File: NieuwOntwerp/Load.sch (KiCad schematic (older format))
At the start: 74 parts, among them J1 Conn_01x02, J2 Conn_01x02, J3 Conn_01x05, J4 Conn_01x03, J5 Conn_01x02, Q1 IRF840, Q2 IRF840, T1 EE13, U1 ESP12E, U10 MCP4725A0, U2 LNK364D, U3 LM358, U4 PC817, U5 TL431, U6 LM1117-3.3, U7 LM358

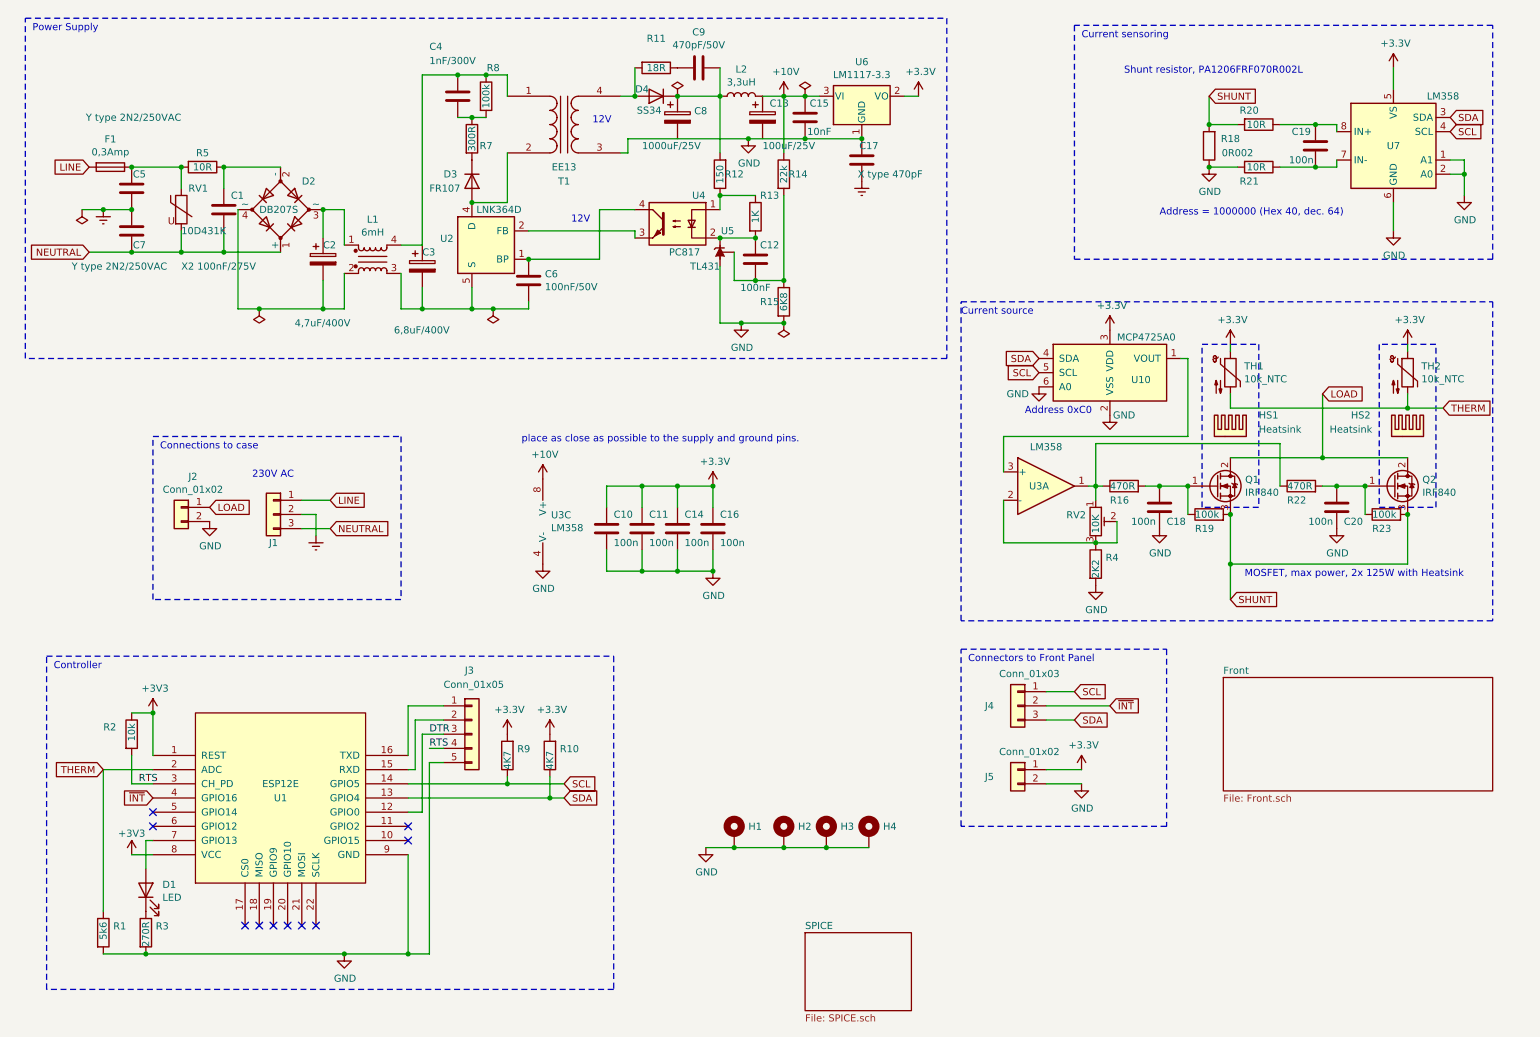
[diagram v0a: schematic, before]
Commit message: Sync_21-04-27
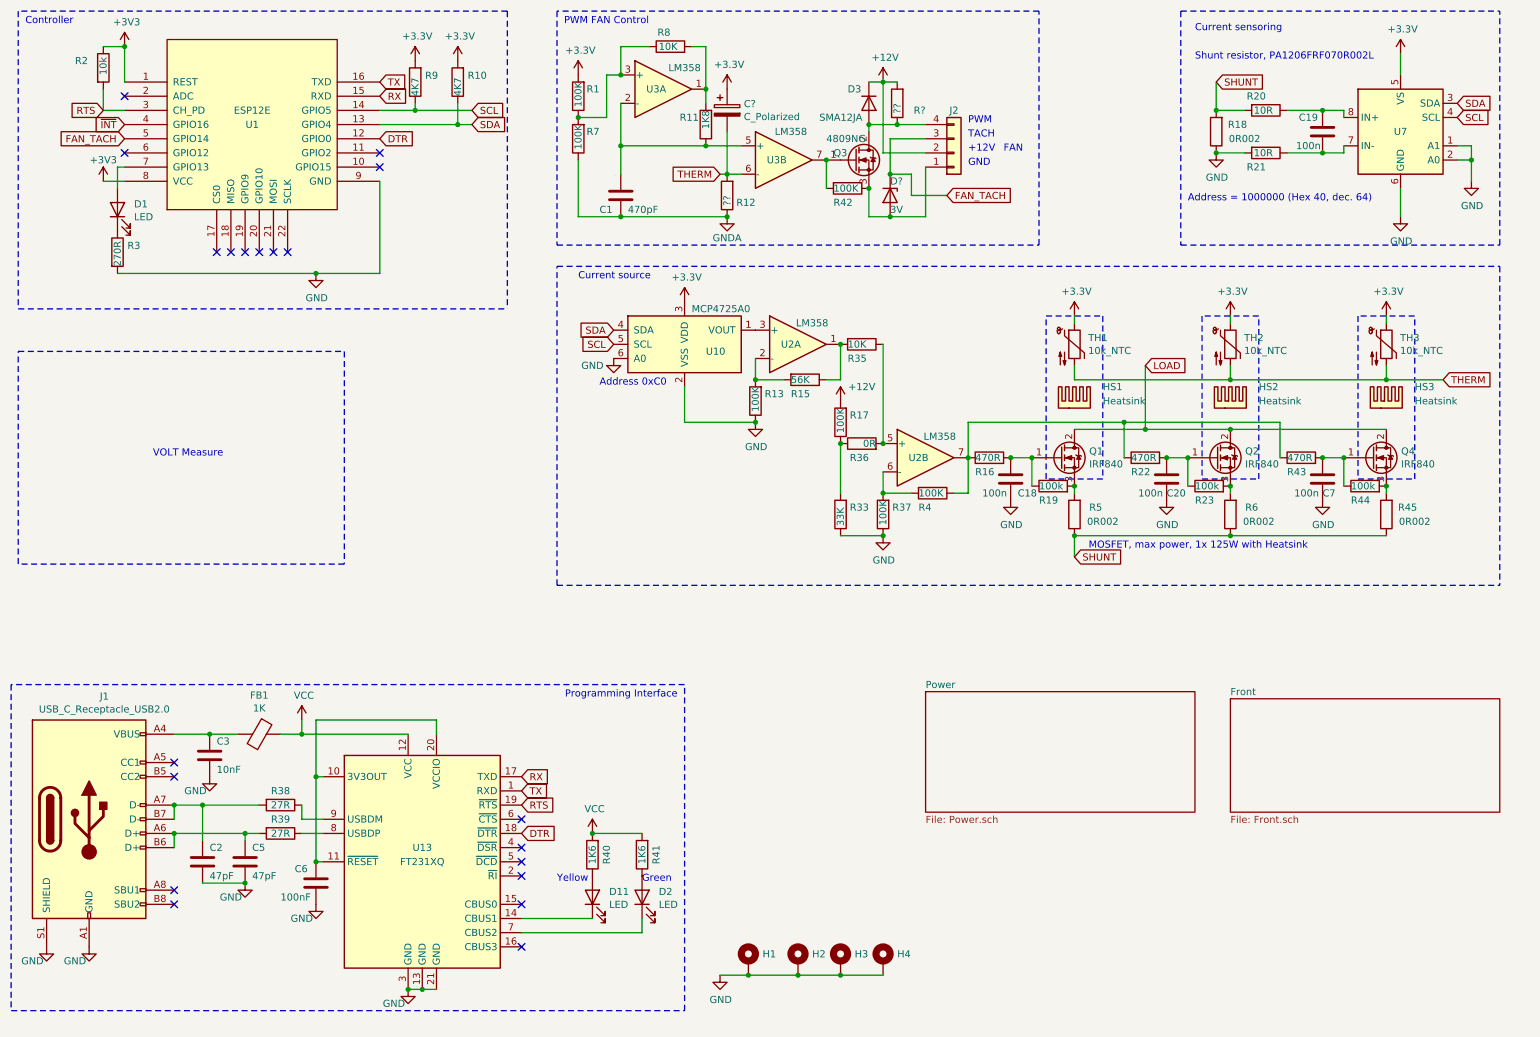
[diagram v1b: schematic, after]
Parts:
- removed C10, C11, C14, C16: 100n, Capacitor_SMD:C_0603_1608Metric, symbol Device:C
- removed C12: 100nF, Capacitor_SMD:C_0603_1608Metric, symbol Device:C
- removed C13: 100uF/25V, Capacitor_THT:CP_Radial_D5.0mm_P2.00mm, symbol Device:C_Polarized
- removed C15: 10nF, Capacitor_SMD:C_0603_1608Metric, symbol Device:C
- removed C17: X type 470pF, Capacitor_SMD:C_0603_1608Metric, symbol Device:C
- removed C2: 4,7uF/400V, Capacitor_THT:CP_Radial_D8.0mm_P3.50mm, symbol Device:C_Polarized
- removed C3: 6,8uF/400V, Capacitor_THT:CP_Radial_D8.0mm_P3.50mm, symbol Device:C_Polarized
- removed C4: 1nF/300V, Condensator:JN_102M, symbol Device:C
- removed C8: 1000uF/25V, Capacitor_THT:CP_Radial_D10.0mm_P5.00mm, symbol Device:C_Polarized
- removed C9: 470pF/50V, Capacitor_SMD:C_0603_1608Metric, symbol Device:C
- removed D2: DB207S, Diode2:SOT4_Rectifier_Bridge, symbol Device:D_Bridge_+-AA
- removed D4: SS34, Diode_SMD:D_SMA, symbol Device:D
- removed F1: 0,3Amp, Fuse:Fuse_1206_3216Metric, symbol Device:Fuse
- removed J1: Conn_01x02, Connector2:JST_XH_B3B-XH-AM_1x03_P2.50mm_Vertical, symbol Connector_Generic:Conn_01x03
- removed J2, J5: Conn_01x02, Connector2:JST_XH_B2B-XH-AM_1x02_P2.50mm_Vertical, symbol Connector_Generic:Conn_01x02
- removed J3: Conn_01x05, Connector2:Molex_PicoBlade_53047-0510_1x05_P1.25mm_Vertical, symbol Connector_Generic:Conn_01x05
- removed J4: Conn_01x03, Connector2:JST_XH_B3B-XH-AM_1x03_P2.50mm_Vertical, symbol Connector_Generic:Conn_01x03
- removed L1: 6mH, Transformers:UU98_Common_Mode_Choke, symbol Device:L_Iron_Coupled_1423
- removed L2: 3,3uH, Inductor_SMD:L_1206_3216Metric, symbol Device:L
- removed R14: 22k, Resistor_SMD:R_0402_1005Metric, symbol Device:R
- removed RV1: 10D431K, Varistor2:RV_Disc_D10mm_W2mm_P8mm, symbol Device:Varistor
- removed RV2: 10K, Potentiometer_THT:Potentiometer_Bourns_3296W_Vertical, symbol Device:R_Potentiometer_Trim
- removed T1: EE13, Transformers:EE13Horizontal, symbol Device:Transformer_1P_1S
- removed U2: LNK364D, Package_SO:PowerIntegrations_SO-8C, symbol Regulator_Switching:LNK364D
- removed unit 3 of U3
- removed U4: PC817, Package_SO:SSO-4_6.7x5.1mm_P2.54mm_Clearance8mm, symbol Isolator:PC817
- removed U5: TL431, Package_TO_SOT_SMD:SOT-23, symbol Reference_Voltage:TL431DBZ
- removed U6: LM1117-3.3, Package_TO_SOT_SMD:SOT-223-3_TabPin2, symbol Regulator_Linear:LM1117-3.3
- added C2: 47pF, Capacitor_SMD:C_0603_1608Metric, symbol Device:C
- added C3: 10nF, Capacitor_SMD:C_0402_1005Metric, symbol Device:C
- added C?: C_Polarized, symbol Device:C_Polarized
- added D11, D2: LED, LED_SMD:LED_0603_1608Metric, symbol Device:LED
- added D?: 3V, symbol Device:D_Zener
- added FB1: 1K, Resistor_SMD:R_0603_1608Metric, symbol Device:FerriteBead
- added HS3: Heatsink, Mechanisch:Heatsink_TO220, symbol Mechanical:Heatsink
- added J1: USB_C_Receptacle_USB2.0, Connector2:USB-C_Receptable_SMD_16pin, symbol Connector:USB_C_Receptacle_USB2.0
- added J2: Conn_01x02, Connector2:JST_XH_B2B-XH-AM_1x02_P2.50mm_Vertical, symbol Connector_Generic:Conn_01x04
- added Q3: 4809NG, Package-SOT:369AA, symbol Device:Q_NMOS_GDS
- added Q4: IRF840, Package_TO_SOT_THT:TO-220-3_Vertical, symbol Device:Q_NMOS_GDS
- added R17, R37, R42: 100K, Resistor_SMD:R_0603_1608Metric, symbol Device:R
- added R33: 33K, Resistor_SMD:R_0603_1608Metric, symbol Device:R
- added R35: 10K, Resistor_SMD:R_0603_1608Metric, symbol Device:R
- added R36: 0R, Resistor_SMD:R_0603_1608Metric, symbol Device:R
- added R38, R39: 27R, Resistor_SMD:R_0603_1608Metric, symbol Device:R
- added R40, R41: 1K6, Resistor_SMD:R_0603_1608Metric, symbol Device:R
- added R43: 470R, Resistor_SMD:R_0603_1608Metric, symbol Device:R
- added R44: 100k, Resistor_SMD:R_0603_1608Metric, symbol Device:R
- added R45, R6: 0R002, Resistor_SMD:R_1206_3216Metric, symbol Device:R
- added R?: ??, Resistor_SMD:R_0603_1608Metric, symbol Device:R
- added TH3: 10k_NTC, Capacitor_THT:C_Disc_D3.8mm_W2.6mm_P2.50mm, symbol Device:Thermistor_NTC
- added U13: FT231XQ, Package_DFN_QFN:QFN-20-1EP_4x4mm_P0.5mm_EP2.5x2.5mm, symbol Interface_USB:FT231XQ
- added unit 1 of U2
- added U3: LM358, Package_SO:SOIC-8_3.9x4.9mm_P1.27mm, symbol Amplifier_Operational:LM358
- C1: value X2 100nF/275V -> 470pF; footprint Condensator:CBB22104J400V -> Capacitor_SMD:C_0402_1005Metric
- C5: value Y type 2N2/250VAC -> 47pF; footprint Condensator:JN_102M -> Capacitor_SMD:C_0603_1608Metric
- C6: value 100nF/50V -> 100nF
- C7: value Y type 2N2/250VAC -> 100n; footprint Condensator:JN_102M -> Capacitor_SMD:C_0603_1608Metric
- D3: value FR107 -> SMA12JA
- R1: value 5k6 -> 100K; footprint Resistor_SMD:R_0603_1608Metric_Pad1.05x0.95mm_HandSolder -> Resistor_SMD:R_0603_1608Metric
- R11: value 18R -> 1K8; footprint Resistor_SMD:R_1206_3216Metric -> Resistor_SMD:R_0603_1608Metric
- R12: value 150 -> ??
- R13: value 1K -> 100K
- R15: value 6K8 -> 56K
- R16, R19, R2, R22, R23, R3: footprint Resistor_SMD:R_0603_1608Metric_Pad1.05x0.95mm_HandSolder -> Resistor_SMD:R_0603_1608Metric
- R4: value 2K2 -> 100K
- R5: value 10R -> 0R002; footprint Resistor_SMD:R_2512_6332Metric -> Resistor_SMD:R_1206_3216Metric
- R7: value 300R -> 100K; footprint Resistor_SMD:R_1210_3225Metric -> Resistor_SMD:R_0603_1608Metric
- R8: value 100k -> 10K; footprint Resistor_SMD:R_1210_3225Metric -> Resistor_SMD:R_0603_1608Metric
- U7: value LM358 -> (none)
- renumbered U3 to U2
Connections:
- net +3V3: now also R1.2, C?.1, TH3.1
- net DTR: now also U13.18 (~DTR)
- net GND: now also C5.2, C6.2, C7.1, R13.1, C2.2, C3.2, J1.A1 (GND), J1.A12 (GND), J1.B1 (GND), J1.B12 (GND), J1.S1 (SHIELD), R33.1, R37.1, U13.13 (GND), U13.21 (GND), U13.3 (GND); no longer R1.2, R15.2, R4.2
- net LOAD: now also Q4.2 (D)
- net RTS: now also U13.19 (~RTS)
- net SHUNT: now also R5.1, R45.1, R6.1; no longer Q1.3 (S), Q2.3 (S), R19.2, R23.2
- net THERM: now also R12.2, C?.2, TH3.2, U3.6 (-); no longer R1.1, U1.2 (ADC)
- net GNDA: now reaches C1.1
- net GNDA: now also R12.1, R7.1; no longer R5.1
- net at R5.2: now also Q1.3 (S), R19.2; no longer C5.2
- net at R8.1: now also R1.1, R7.2, U3.3 (+)
- net at C6.1: now also U13.10 (3V3OUT), U13.11 (~RESET), U13.20 (VCCIO)
- net at D3.2 (A): now also J2.4 (Pin_4), Q3.2 (D), R?.1
- net at R13.2: now also R15.2, U2.2 (-)
- net at R11.2: now also R8.2, U3.1
- net at R15.1: now also R35.2, U2.1
- net +12V: now reaches D3.1 (K)
- net +12V: now also J2.2 (Pin_2), R17.2, R?.2; no longer R7.2
- net at R11.1: now also C1.2, U3.2 (-), U3.5 (+)
- net at R16.1, R22.1: now also R4.1, U2.7, R43.1; no longer U2.1
- net at U10.1 (VOUT): now also U2.3 (+); no longer U2.3 (+)
- net TX: now reaches U1.16 (TXD)
- net TX: now also U13.1 (RXD)
- net RX: now reaches U1.15 (RXD)
- net RX: now also U13.17 (TXD)
- net FAN_TACH: now reaches U1.5 (GPIO14)
- net FAN_TACH: now also D?.1 (K), J2.3 (Pin_3)
- net Earth: no longer names the net of C5.1
- net Earth: now also J1.A6 (D+), J1.B6 (D+), R39.2; no longer C7.2
- removed net NEUTRAL: C1.2, C7.1
- new net: R35.1, R36.2, U2.5 (+)
- new net: R37.2, R4.2, U2.6 (-)
- new net: Q2.3 (S), R23.2, R6.2
- new net: C3.1, FB1.2, J1.A4 (VBUS), J1.A9 (VBUS), J1.B4 (VBUS), J1.B9 (VBUS)
- new net: C2.1, J1.A7 (D-), J1.B7 (D-), R38.2
- new net: D11.1 (K), U13.14 (CBUS1)
- new net: D2.1 (K), U13.7 (CBUS2)
- new net: R39.1, U13.8 (USBDP)
- new net: R38.1, U13.9 (USBDM)
- new net: D11.2 (A), R40.1
- new net: D2.2 (A), R41.1
- new net: C7.2, Q4.1 (G), R43.2, R44.1
- new net: Q4.3 (S), R44.2, R45.2
- new net: R17.1, R33.2, R36.1
- new net: Q3.1 (G), R42.2, U3.7
- new net: D?.2 (A), J2.1 (Pin_1), Q3.3 (S), R42.1
- new net VCC: FB1.1, R40.2, R41.2, U13.12 (VCC)
- no-connect marks 10 -> 20
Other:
- note added: "+12V"
- note added: "FAN"
- note added: "GND"
- note added: "Green"
- note added: "MOSFET, max power, 1x 125W with Heatsink"
- note added: "PWM"
- note added: "PWM FAN Control"
- note added: "Programming Interface"
- note added: "TACH"
- note added: "VOLT Measure"
- note added: "Yellow"
- note removed: "12V"
- note removed: "230V AC"
- note removed: "Connections to case"
- note removed: "Connectors to Front Panel"
- note removed: "MOSFET, max power, 2x 125W with Heatsink"
- note removed: "Power Supply"
- note removed: "place as close as possible to the supply and ground pins."
- moved on the sheet: C18, C19, C20, D1, H1, H2, H3, H4, HS1, HS2, Q1, Q2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

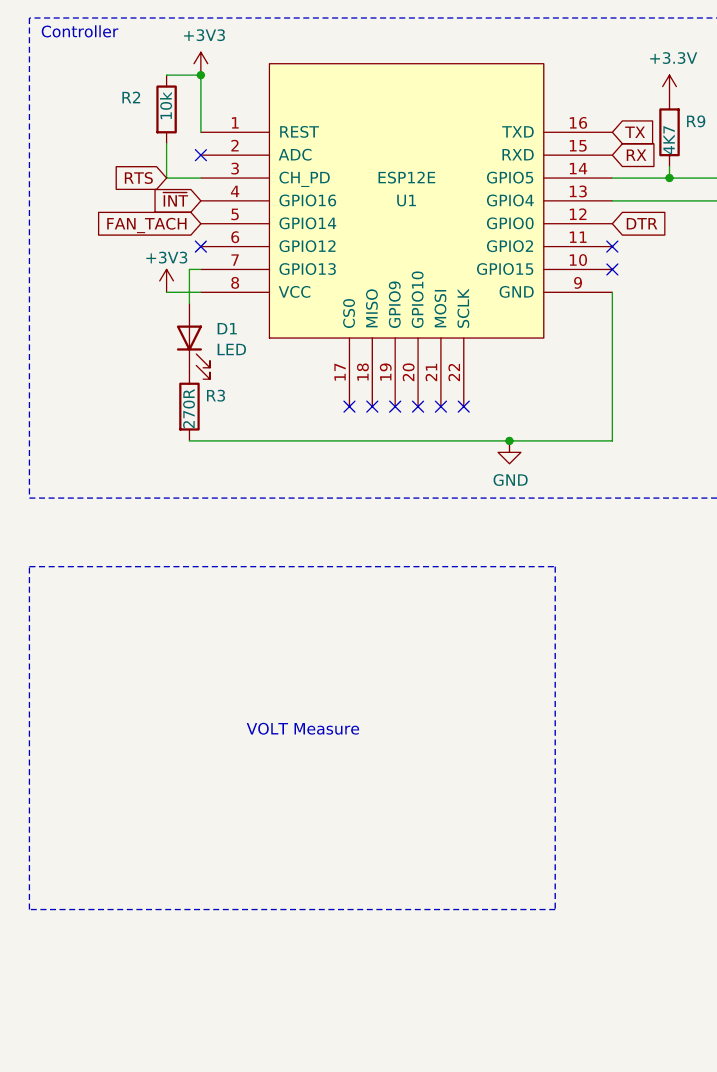
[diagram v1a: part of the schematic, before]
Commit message: 2021-04-27_02
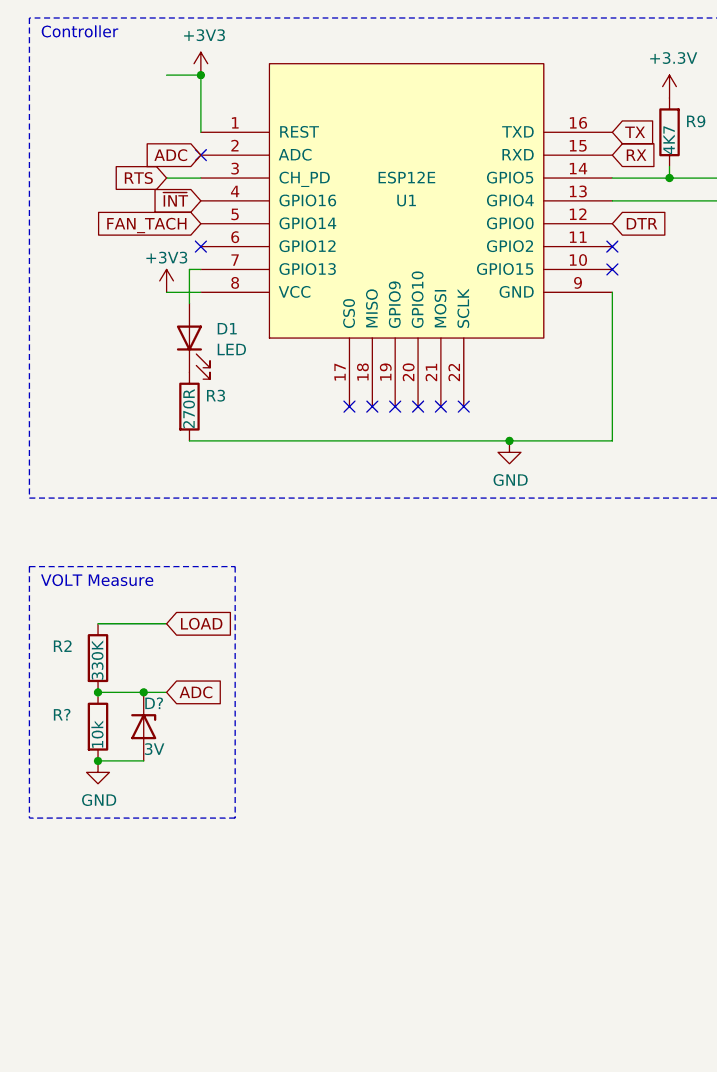
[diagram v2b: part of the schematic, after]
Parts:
- added D?: 3V, symbol Device:D_Zener
- added R?: 10k, Resistor_SMD:R_0603_1608Metric, symbol Device:R
- R2: value 10k -> 330K
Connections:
- net +3V3: no longer R2.1
- net GND: now also D?.2 (A), R?.2
- net LOAD: now also R2.1
- net RTS: no longer R2.2
- net ADC: now reaches U1.2 (ADC)
- net ADC: now also R2.2, D?.1 (K), R?.1
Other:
- moved on the sheet: R2
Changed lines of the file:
@@
 L Device:R R2
 U 1 1 6015AC04
-P 1200 1050
-F 0 "R2" H 1000 1100 50  0000 L CNN
-F 1 "10k" V 1200 1000 50  0000 L CNN
-F 2 "Resistor_SMD:R_0603_1608Metric" V 1130 1050 50  0001 C CNN
-F 3 "~" H 1200 1050 50  0001 C CNN
-	1    1200 1050
-	1    0    0    -1
-$EndComp
-Wire Wire Line
-	1200 1200 1200 1350
+P 900 3450
+F 0 "R2" H 700 3500 50  0000 L CNN
+F 1 "330K" V 900 3350 50  0000 L CNN
+F 2 "Resistor_SMD:R_0603_1608Metric" V 830 3450 50  0001 C CNN
+F 3 "~" H 900 3450 50  0001 C CNN
+	1    900  3450
+	1    0    0    -1
+$EndComp
 Wire Wire Line
 	1350 1150 1350 900
@@
 Wire Notes Line
 	4400 4700 11050 4700
-Wire Notes Line
-	600  3050 2900 3050
-Wire Notes Line
-	2900 3050 2900 4550
-Wire Notes Line
-	2900 4550 600  4550
-Wire Notes Line
-	600  4550 600  3050
-Text Notes 1550 3800 0    50   ~ 0
+Text Notes 650  3150 0    50   ~ 0
 VOLT Measure
 Wire Wire Line
@@
 Connection ~ 5450 1200
 Connection ~ 6300 1700
+$Comp
+L Device:R R?
+U 1 1 6088EF1E
+P 900 3750
+F 0 "R?" H 700 3800 50  0000 L CNN
+F 1 "10k" V 900 3650 50  0000 L CNN
+F 2 "Resistor_SMD:R_0603_1608Metric" V 830 3750 50  0001 C CNN
+F 3 "~" H 900 3750 50  0001 C CNN
+	1    900  3750
+	1    0    0    -1
+$EndComp
+Text GLabel 1200 3600 2    50   Input ~ 0
+ADC
+Text GLabel 1350 1250 0    50   Input ~ 0
+ADC
+$Comp
+L Device:D_Zener D?
+U 1 1 6088FDD6
+P 1100 3750
+F 0 "D?" V 1000 3750 50  0000 L CNN
+F 1 "3V" V 1200 3750 50  0000 L CNN
+F 2 "" H 1100 3750 50  0001 C CNN
+F 3 "~" H 1100 3750 50  0001 C CNN
+	1    1100 3750
+	0    1    1    0
+$EndComp
+$Comp
+L power:GND #PWR?
+U 1 1 60890C03
+P 900 3900
+F 0 "#PWR?" H 900 3650 50  0001 C CNN
+F 1 "GND" H 905 3727 50  0000 C CNN
+F 2 "" H 900 3900 50  0001 C CNN
+F 3 "" H 900 3900 50  0001 C CNN
+	1    900  3900
+	1    0    0    -1
+$EndComp
+Wire Wire Line
+	1200 3600 1100 3600
+Connection ~ 900  3600
+Connection ~ 1100 3600
+Wire Wire Line
+	1100 3600 900  3600
+Text GLabel 1200 3300 2    50   Input ~ 0
+LOAD
+Wire Wire Line
+	1200 3300 900  3300
+Wire Wire Line
+	1100 3900 900  3900
+Connection ~ 900  3900
+Wire Notes Line
+	600  3050 1500 3050
+Wire Notes Line
+	1500 3050 1500 4150
+Wire Notes Line
+	1500 4150 600  4150
+Wire Notes Line
+	600  3050 600  4150
 $EndSCHEMATC
